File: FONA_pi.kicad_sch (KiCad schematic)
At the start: 21 parts, among them J1 Conn_01x20_Socket, J10 Conn_01x04_Pin, J11 Conn_01x20_Socket, J12 Conn_01x20_Socket, J2 Conn_02x20_Odd_Even, J3 Conn_01x20_Socket, J4 Conn_01x20_Socket, J5 Conn_01x18, J6 Conn_01x18_Socket, J7 Conn_01x20_Socket, J8 Conn_01x18, J9 Conn_01x04_Pin

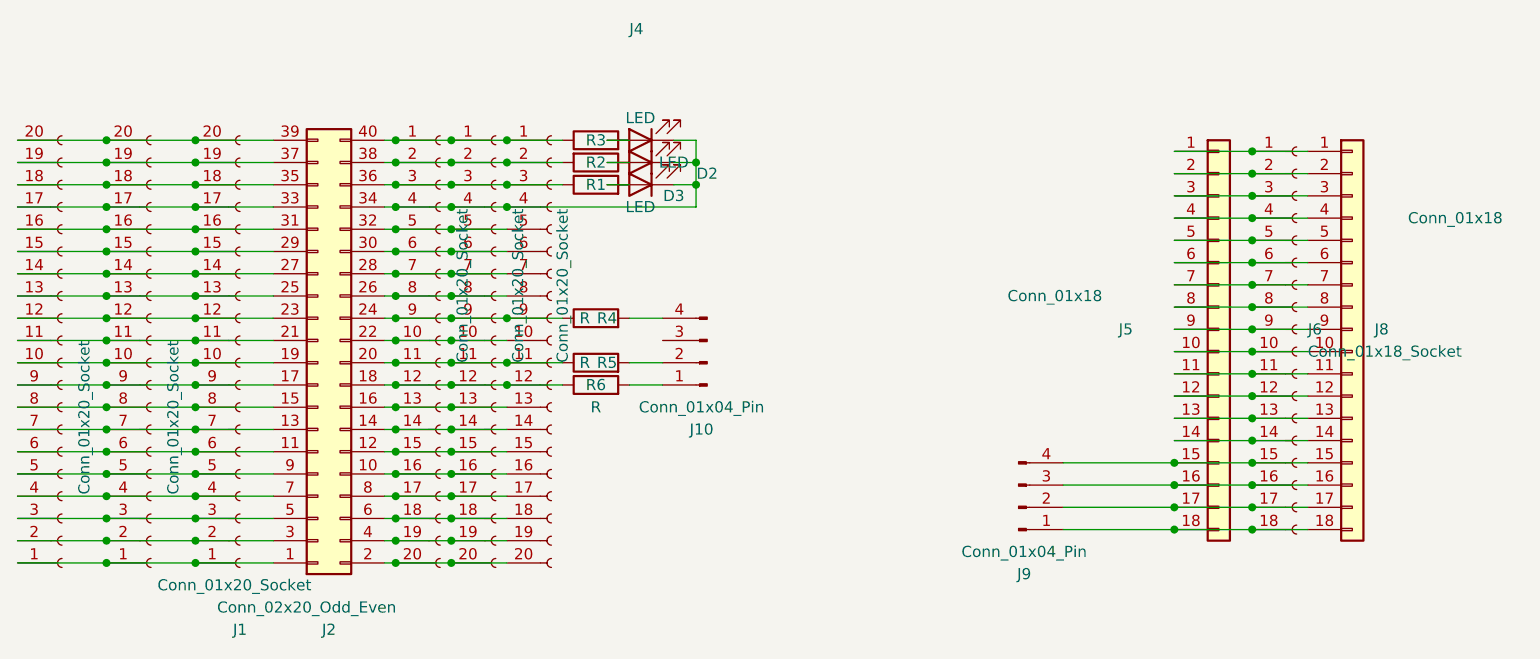
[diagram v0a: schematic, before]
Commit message: tweaks after running DRC
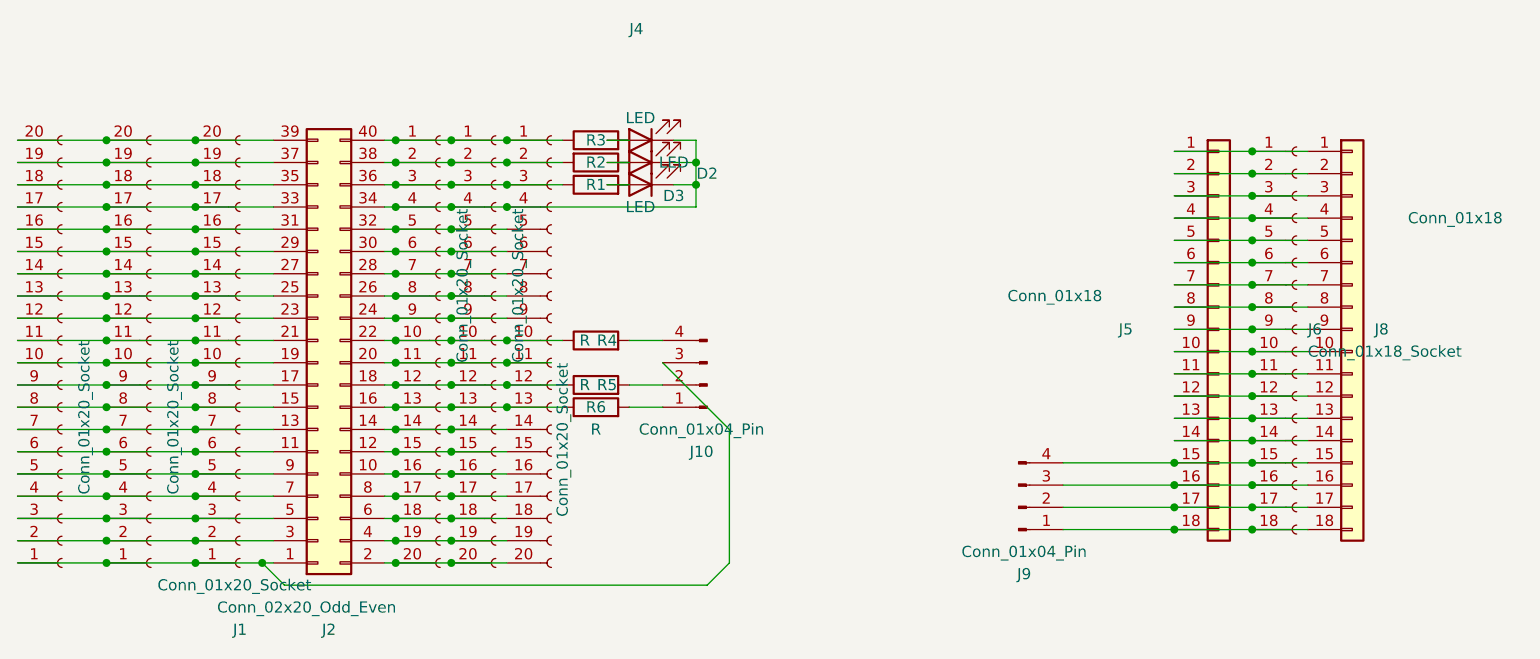
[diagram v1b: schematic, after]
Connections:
- net at J2.22 (Pin_22), J3.10 (Pin_10), J4.10 (Pin_10)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: now also R4.1
- net at J2.20 (Pin_20), J3.11 (Pin_11), J4.11 (Pin_11)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: no longer R5.1
- net at J2.18 (Pin_18), J3.12 (Pin_12), J4.12 (Pin_12)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: now also R5.1; no longer R6.1
- net at J2.16 (Pin_16), J3.13 (Pin_13), J4.13 (Pin_13)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: now also R6.1
- net at J2.24 (Pin_24), J3.9 (Pin_9), J4.9 (Pin_9)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: no longer R4.1
- net at J1.1 (Pin_1), J11.1 (Pin_1), J12.1 (Pin_1)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: now also J10.3 (Pin_3)
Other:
- moved on the sheet: J10, R4, R5, R6
